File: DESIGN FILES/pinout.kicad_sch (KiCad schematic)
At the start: 1 part, among them U701 M.2-B-KEY

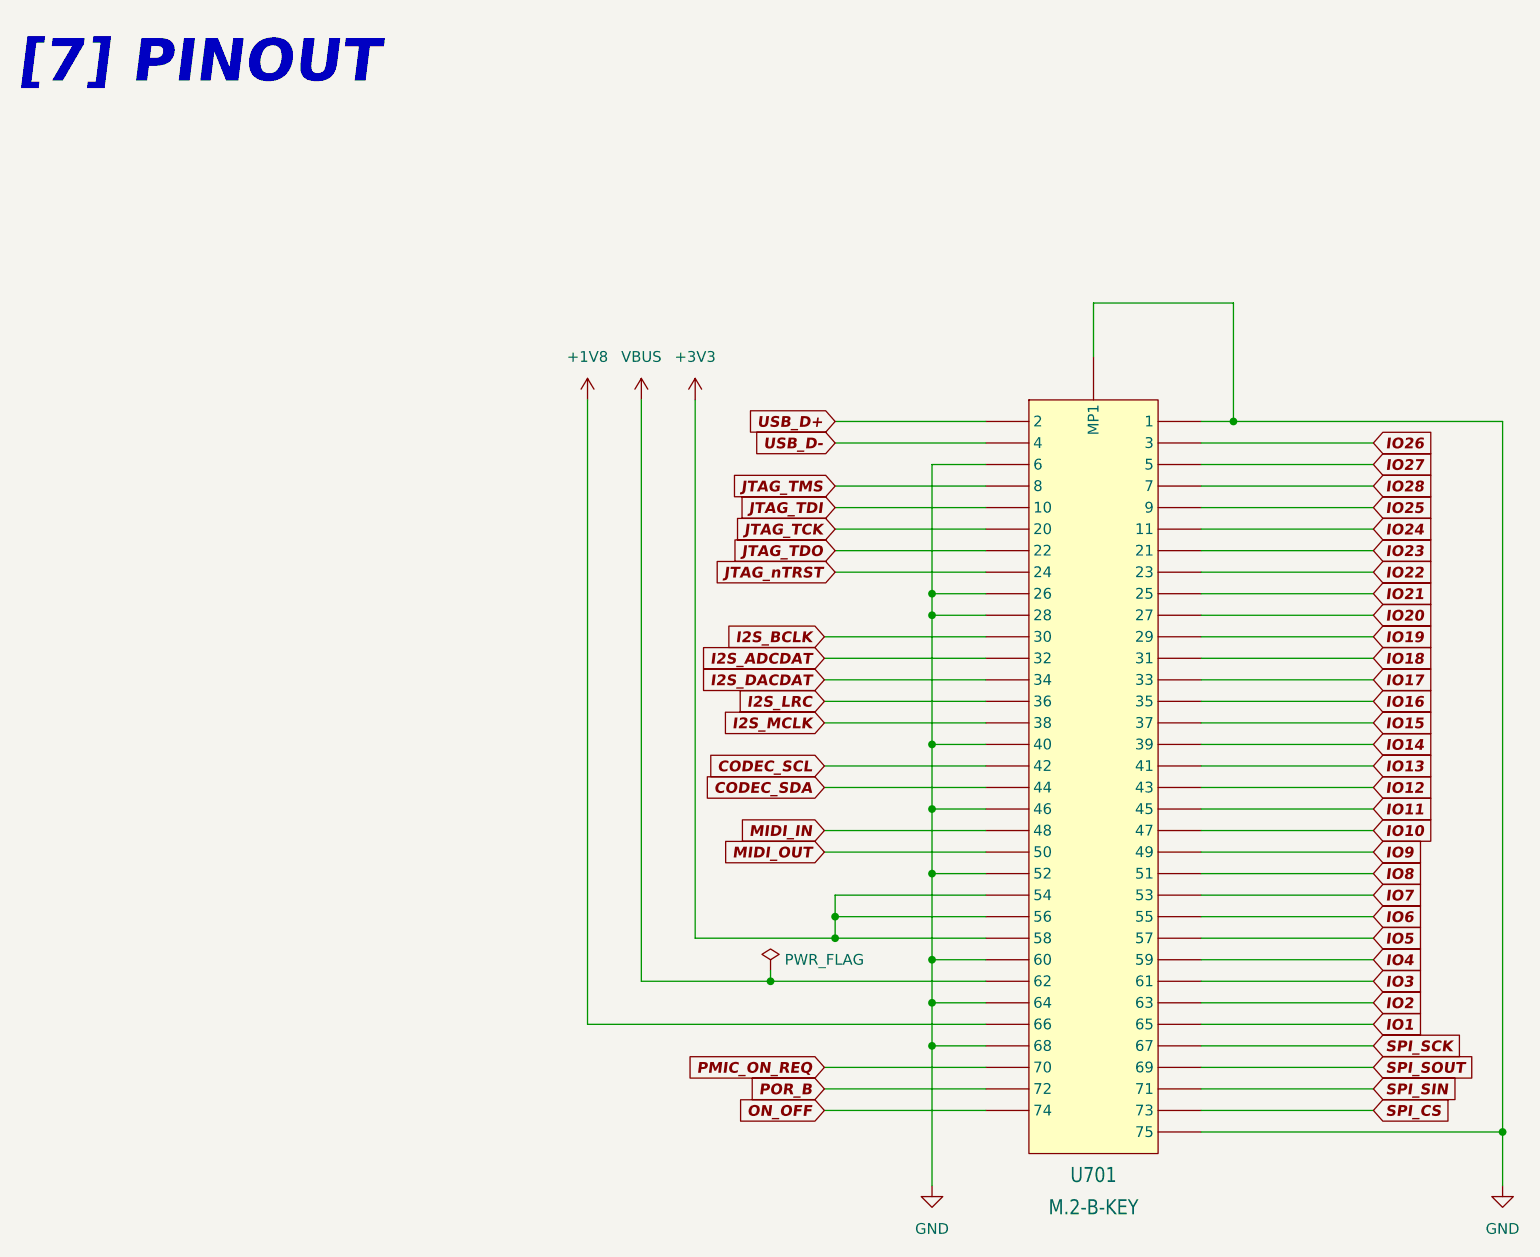
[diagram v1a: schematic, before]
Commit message: up
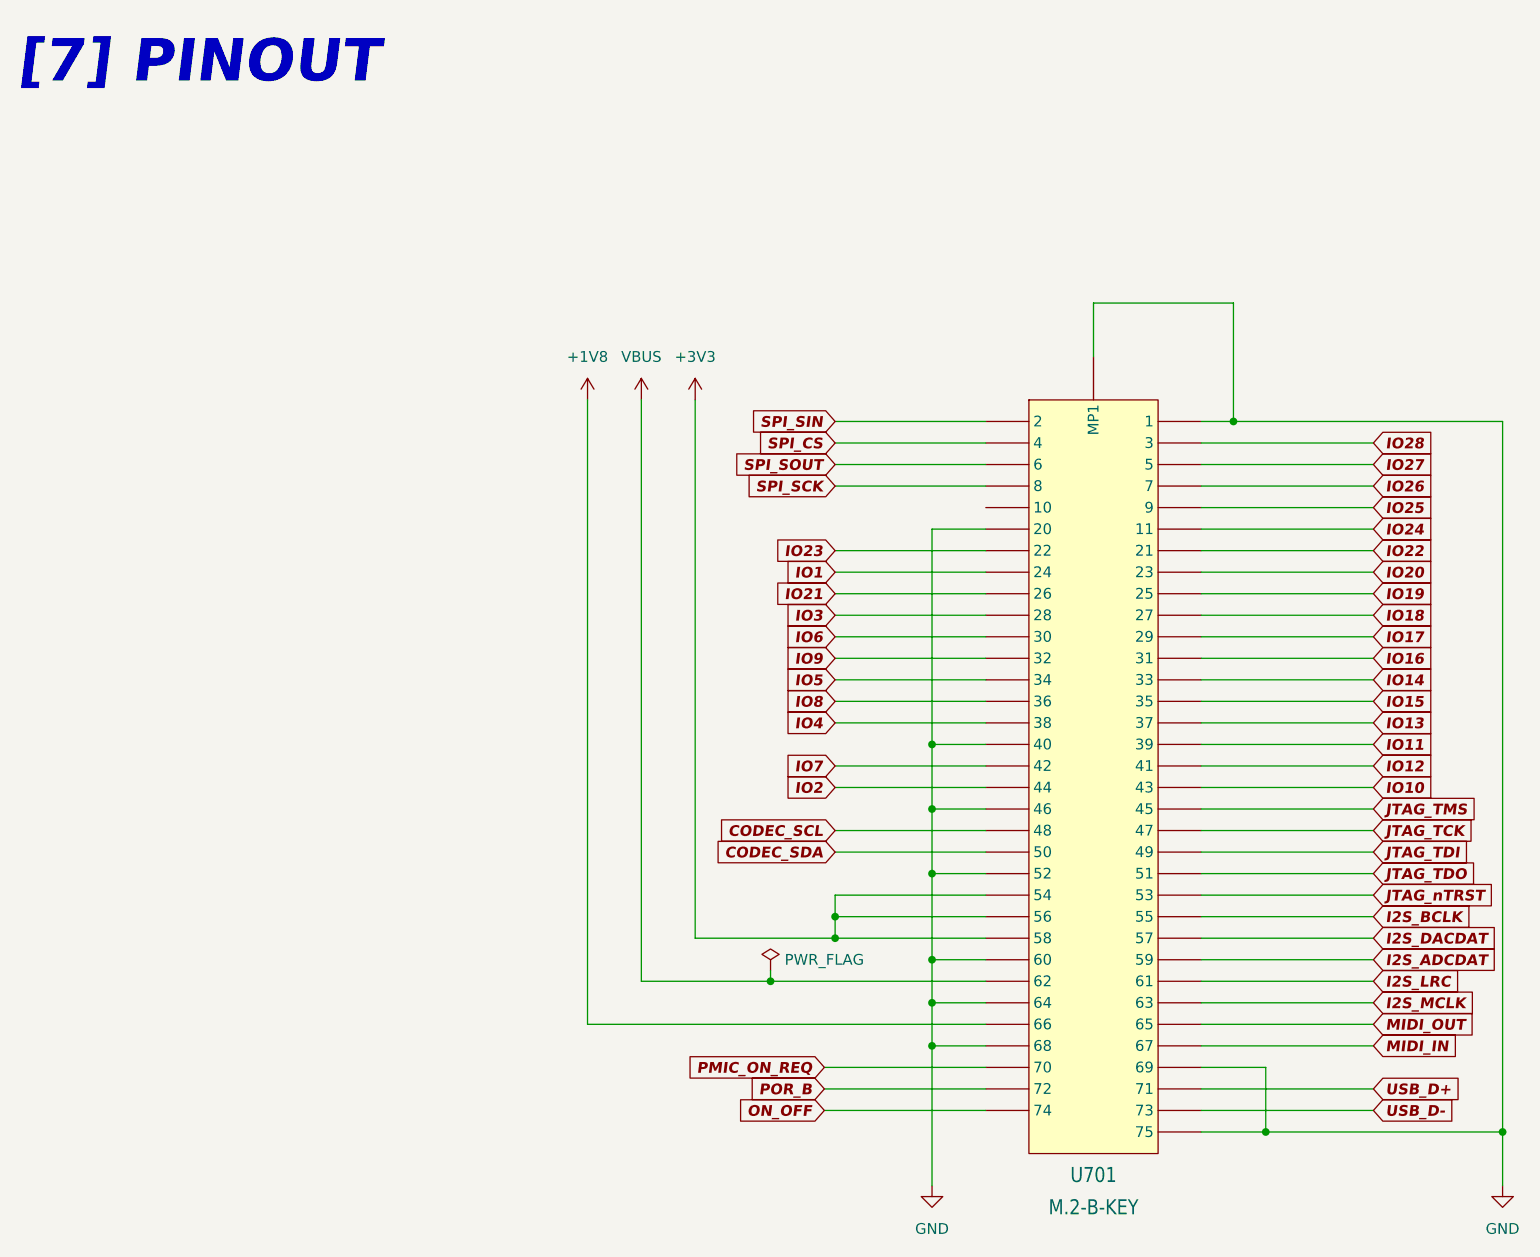
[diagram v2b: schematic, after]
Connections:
- net CODEC_SCL: now also U701.P$48 (48); no longer U701.P$42 (42)
- net CODEC_SDA: now also U701.P$50 (50); no longer U701.P$44 (44)
- net GND: now also U701.P$20 (20), U701.P$69 (69); no longer U701.P$26 (26), U701.P$28 (28), U701.P$6 (6)
- net I2S_ADCDAT: now also U701.P$59 (59); no longer U701.P$32 (32)
- net I2S_BCLK: now also U701.P$55 (55); no longer U701.P$30 (30)
- net I2S_DACDAT: now also U701.P$57 (57); no longer U701.P$34 (34)
- net I2S_LRC: now also U701.P$61 (61); no longer U701.P$36 (36)
- net I2S_MCLK: now also U701.P$63 (63); no longer U701.P$38 (38)
- net IO1: now also U701.P$24 (24); no longer U701.P$65 (65)
- net IO10: now also U701.P$43 (43); no longer U701.P$47 (47)
- net IO11: now also U701.P$39 (39); no longer U701.P$45 (45)
- net IO12: now also U701.P$41 (41); no longer U701.P$43 (43)
- net IO13: now also U701.P$37 (37); no longer U701.P$41 (41)
- net IO14: now also U701.P$33 (33); no longer U701.P$39 (39)
- net IO15: now also U701.P$35 (35); no longer U701.P$37 (37)
- net IO16: now also U701.P$31 (31); no longer U701.P$35 (35)
- net IO17: now also U701.P$29 (29); no longer U701.P$33 (33)
- net IO18: now also U701.P$27 (27); no longer U701.P$31 (31)
- net IO19: now also U701.P$25 (25); no longer U701.P$29 (29)
- net IO2: now also U701.P$44 (44); no longer U701.P$63 (63)
- net IO20: now also U701.P$23 (23); no longer U701.P$27 (27)
- net IO21: now also U701.P$26 (26); no longer U701.P$25 (25)
- net IO22: now also U701.P$21 (21); no longer U701.P$23 (23)
- net IO23: now also U701.P$22 (22); no longer U701.P$21 (21)
- net IO26: now also U701.P$7 (7); no longer U701.P$3 (3)
- net IO28: now also U701.P$3 (3); no longer U701.P$7 (7)
- net IO3: now also U701.P$28 (28); no longer U701.P$61 (61)
- net IO4: now also U701.P$38 (38); no longer U701.P$59 (59)
- net IO5: now also U701.P$34 (34); no longer U701.P$57 (57)
- net IO6: now also U701.P$30 (30); no longer U701.P$55 (55)
- net IO7: now also U701.P$42 (42); no longer U701.P$53 (53)
- net IO8: now also U701.P$36 (36); no longer U701.P$51 (51)
- net IO9: now also U701.P$32 (32); no longer U701.P$49 (49)
- net JTAG_TCK: now also U701.P$47 (47); no longer U701.P$20 (20)
- net JTAG_TDI: now also U701.P$49 (49); no longer U701.P$10 (10)
- net JTAG_TDO: now also U701.P$51 (51); no longer U701.P$22 (22)
- net JTAG_TMS: now also U701.P$45 (45); no longer U701.P$8 (8)
- net JTAG_nTRST: now also U701.P$53 (53); no longer U701.P$24 (24)
- net MIDI_IN: now also U701.P$67 (67); no longer U701.P$48 (48)
- net MIDI_OUT: now also U701.P$65 (65); no longer U701.P$50 (50)
- net SPI_CS: now also U701.P$4 (4); no longer U701.P$73 (73)
- net SPI_SCK: now also U701.P$8 (8); no longer U701.P$67 (67)
- net SPI_SIN: now also U701.P$2 (2); no longer U701.P$71 (71)
- net SPI_SOUT: now also U701.P$6 (6); no longer U701.P$69 (69)
- net USB_D+: now also U701.P$71 (71); no longer U701.P$2 (2)
- net USB_D-: now also U701.P$73 (73); no longer U701.P$4 (4)
